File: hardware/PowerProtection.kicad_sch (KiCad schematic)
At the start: 17 parts, among them U7 LM76202QPWPRQ1

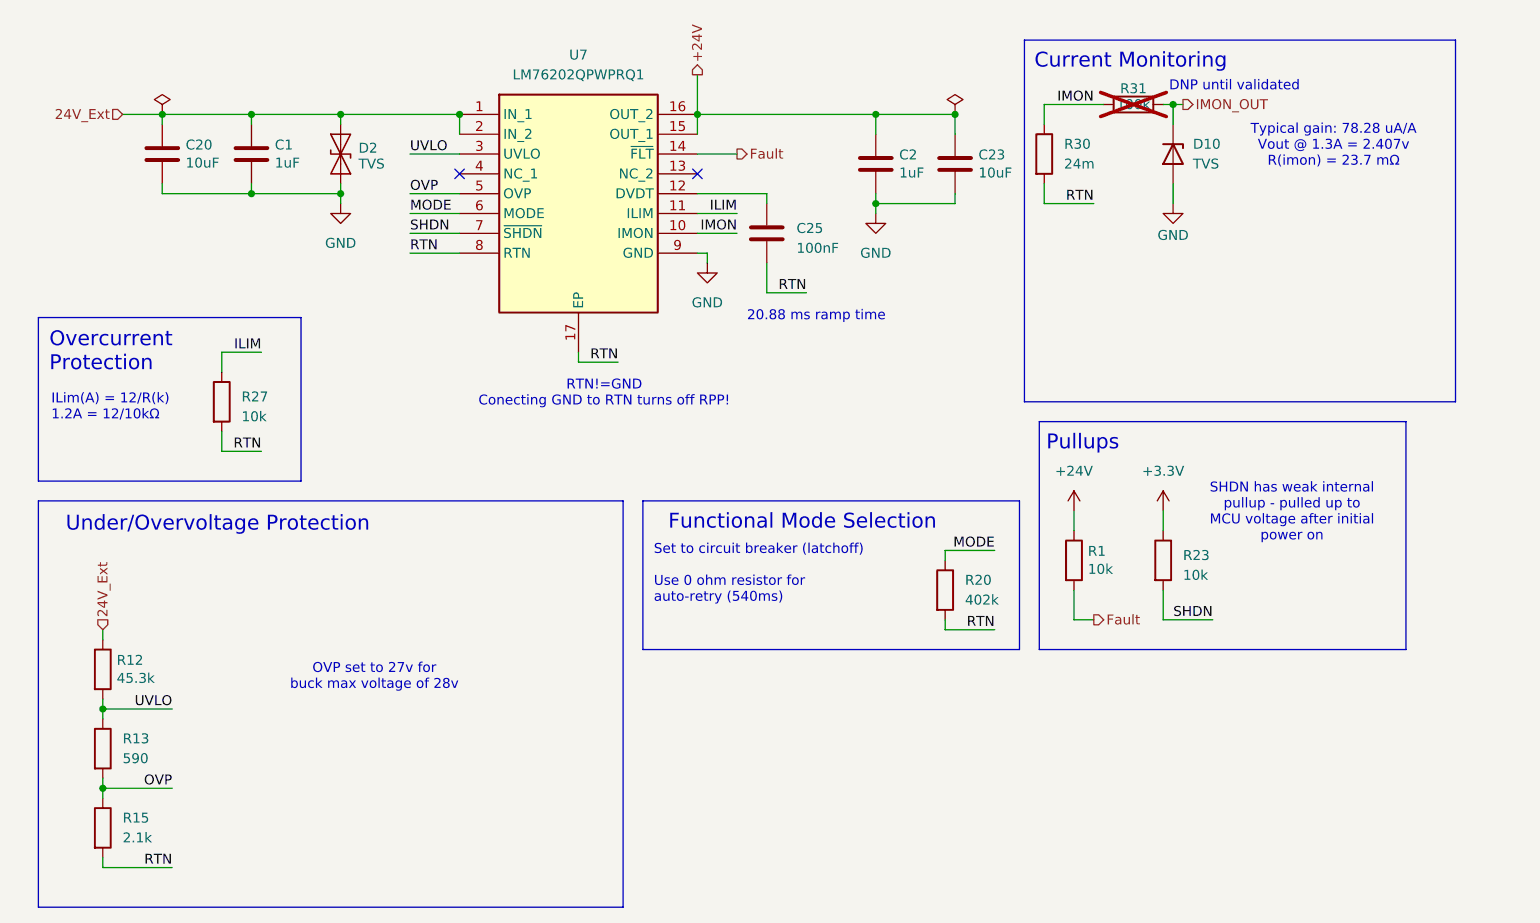
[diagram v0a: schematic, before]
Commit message: added calcs, cleaned up, addressed comments
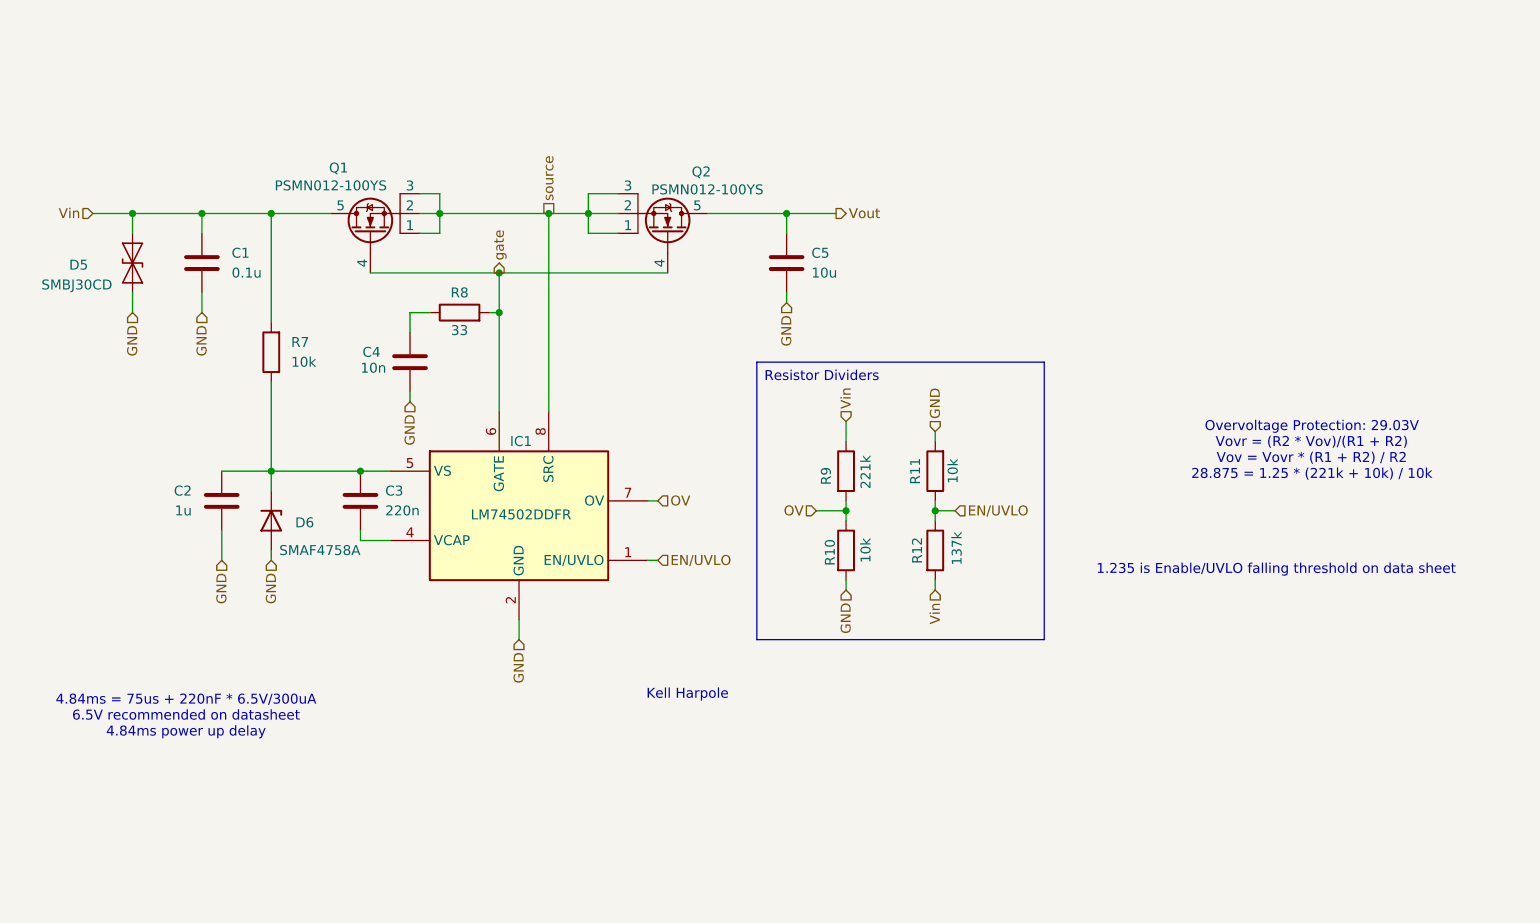
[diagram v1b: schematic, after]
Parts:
- removed C20, C23: 10uF, Capacitor_SMD:C_0805_2012Metric_Pad1.18x1.45mm_HandSolder, symbol Device:C
- removed C25: 100nF, Capacitor_SMD:C_0603_1608Metric_Pad1.08x0.95mm_HandSolder, symbol Device:C
- removed D10: TVS, Diode_SMD:D_SOD-123F, symbol Device:D_Zener
- removed D2: TVS, Diode_SMD:D_SOD-323_HandSoldering, symbol Diode:SD12_SOD323
- removed R1, R23, R27: 10k, Resistor_SMD:R_0603_1608Metric_Pad0.98x0.95mm_HandSolder, symbol Device:R
- removed R13: 590, Resistor_SMD:R_0603_1608Metric_Pad0.98x0.95mm_HandSolder, symbol Device:R
- removed R15: 2.1k, Resistor_SMD:R_0603_1608Metric_Pad0.98x0.95mm_HandSolder, symbol Device:R
- removed R20: 402k, Resistor_SMD:R_0603_1608Metric_Pad0.98x0.95mm_HandSolder, symbol Device:R
- removed R30: 24m, Resistor_SMD:R_0603_1608Metric_Pad0.98x0.95mm_HandSolder, symbol Device:R
- removed R31: 100k, Resistor_SMD:R_0603_1608Metric_Pad0.98x0.95mm_HandSolder, symbol Device:R
- removed U7: LM76202QPWPRQ1, LHRS_Power:LM76202QPWPRQ1, symbol lhrs_power:LM76202QPWPRQ1
- added C3: 220n, Capacitor_SMD:C_0603_1608Metric_Pad1.08x0.95mm_HandSolder, symbol Device:C
- added C4: 10n, Capacitor_SMD:C_0603_1608Metric_Pad1.08x0.95mm_HandSolder, symbol ECE319H:C
- added C5: 10u, Capacitor_SMD:C_0805_2012Metric_Pad1.18x1.45mm_HandSolder, symbol Device:C
- added D5: SMBJ30CD, Diode_SMD:D_SMB, symbol Device:D_Zener
- added D6: SMAF4758A, LHRS_Passives:SODFL5026X125N, symbol Device:D_Zener
- added IC1: LM74502DDFR, LHRS_Power:LM74502DDFR, symbol LHRS_ICs:LM74502HDDFR
- added Q1, Q2: PSMN012-100YS, Package_TO_SOT_SMD:LFPAK56, symbol lhrs_power:PSMN012-100YS
- added R10, R11, R7: 10k, Resistor_SMD:R_0603_1608Metric_Pad0.98x0.95mm_HandSolder, symbol Device:R
- added R8: 33, Resistor_SMD:R_0603_1608Metric_Pad0.98x0.95mm_HandSolder, symbol Device:R
- added R9: 221k, Resistor_SMD:R_0603_1608Metric_Pad0.98x0.95mm_HandSolder, symbol Device:R
- C1: value 1uF -> 0.1u; LCSC P/N (none) -> C14663; P/N MLASU168SB5105KTNA01 -> MLASH168SB7104KTNA01
- C2: value 1uF -> 1u; LCSC P/N (none) -> C15849
- R12: value 45.3k -> 137k; LCSC P/N (none) -> C2090646; P/N CRCW060345K3FKEAHP -> CRCW0603137KFKEA
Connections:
- net +24V is gone; now on net GND: C2.1
- net GND: now also C4.2, C5.2, D5.2 (A2), D6.2 (A), IC1.2 (GND), R10.2, R11.2; no longer C2.2
- net 24V_Ext renamed EN/UVLO
- net EN/UVLO: now also IC1.1 (EN/UVLO), R11.1; no longer C1.1
- net UVLO renamed Vin
- net Vin: now also C1.1, D5.1 (A1), Q1.5, R7.2, R9.1
- new net: C2.2, C3.1, D6.1 (K), IC1.5 (VS), R7.1
- new net: C3.2, IC1.4 (VCAP)
- new net: C4.1, R8.1
- new net OV: IC1.7 (OV), R10.1, R9.2
- new net Vout: C5.1, Q2.5
- new net gate: IC1.6 (GATE), Q1.4, Q2.4, R8.2
- new net source: IC1.8 (SRC), Q1.1, Q1.2, Q1.3, Q2.1, Q2.2, Q2.3
- no-connect marks 2 -> 0
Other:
- note added: "1.235 is Enable/UVLO falling threshold on data sheet"
- note added: "4.84ms = 75us + 220nF * 6.5V/300uA 6.5V recommended on datasheet 4.84ms power up delay"
- note added: "Kell Harpole"
- note added: "Overvoltage Protection: 29.03V Vovr = (R2 * Vov)/(R1 + R2) Vov = Vovr * (R1 + R2) / R2 28.875 = 1.25 * (221k + 10k) / 10k"
- note removed: "20.88 ms ramp time"
- note removed: "Current Monitoring"
- note removed: "DNP until validated"
- note removed: "Functional Mode Selection"
- note removed: "ILim(A) = 12/R(k) 1.2A = 12/10kΩ"
- note removed: "OVP set to 27v for buck max voltage of 28v"
- note removed: "Overcurrent Protection"
- note removed: "Pullups"
- note removed: "RTN!=GND Conecting GND to RTN turns off RPP!"
- note removed: "SHDN has weak internal pullup - pulled up to MCU voltage after initial power on"
- note removed: "Set to circuit breaker (latchoff) Use 0 ohm resistor for auto-retry (540ms)"
- note removed: "Typical gain: 78.28 uA/A Vout @ 1.3A = 2.407v R(imon) = 23.7 mΩ"
- note removed: "Under/Overvoltage Protection"
